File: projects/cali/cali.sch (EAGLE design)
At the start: 25 parts, among them T1 IRLML2502, T2 IRLML2502, T3 2N7002E, T4 IRLML2502

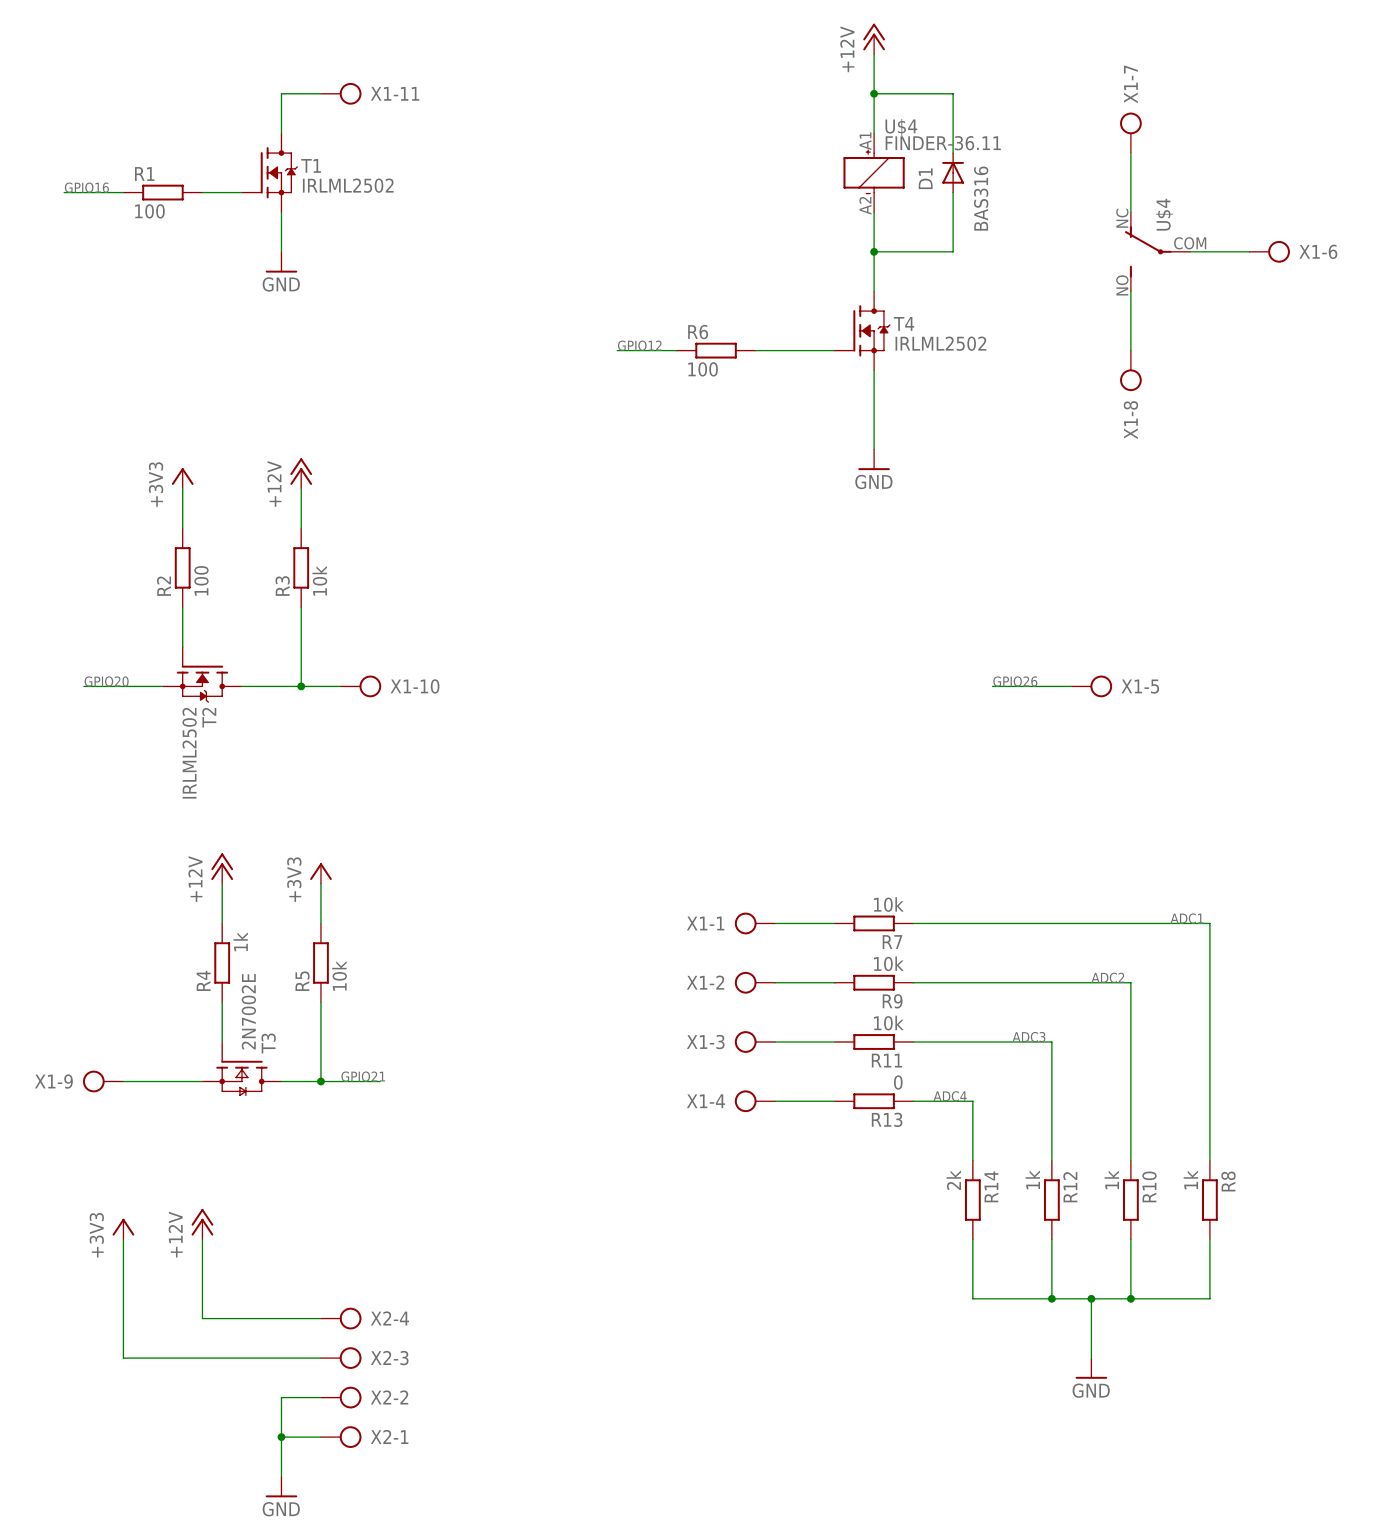
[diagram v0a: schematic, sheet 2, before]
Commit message: Caliboard 1.0 routing done
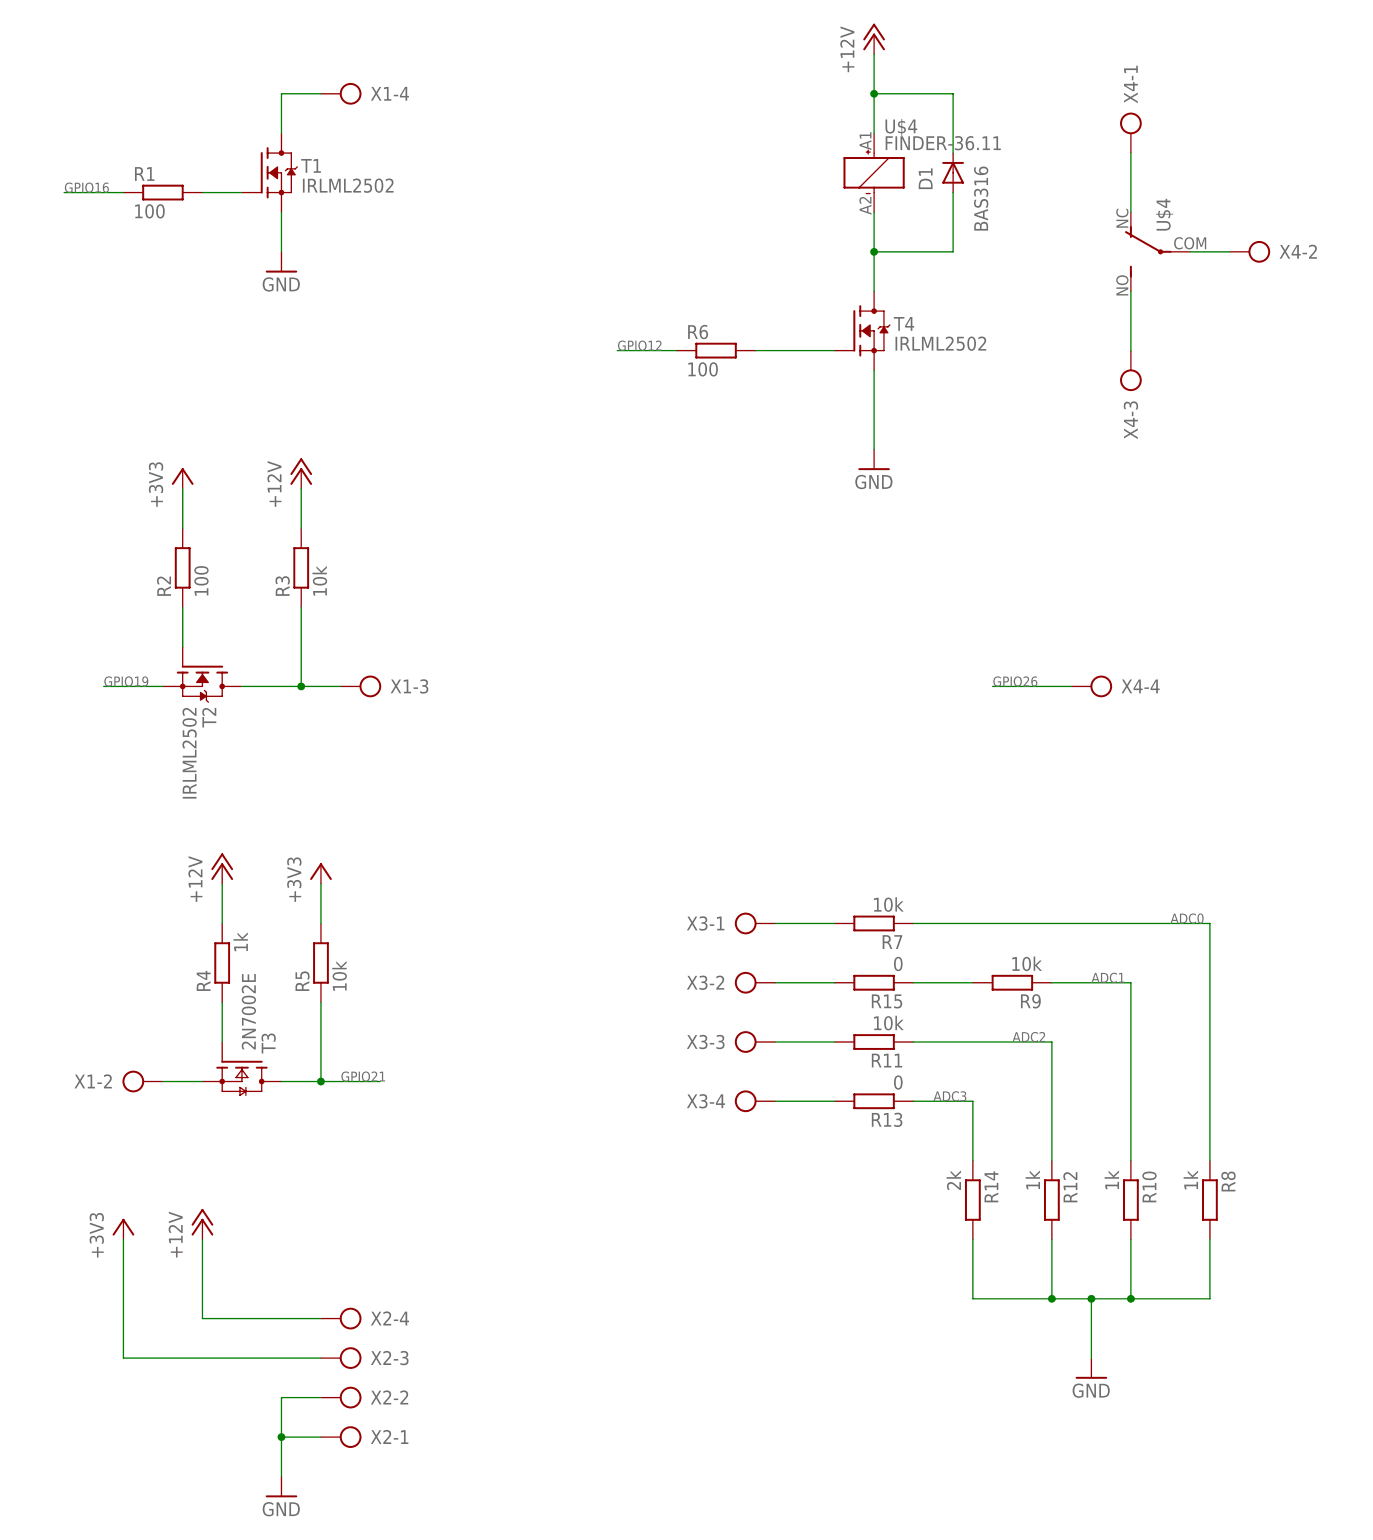
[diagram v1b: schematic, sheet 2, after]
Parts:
- added R15: 0, rcl:R-EU_R1206
- added X3, X4: (no value), con-ptr500:AK500/4
- X1: device con-ptr500:AK500/12 -> con-ptr500:AK500/4
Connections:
- removed net ADC4: R13.1, R14.1
- removed net N$14: R11.2, X1-3.KL
- removed net N$15: R13.2, X1-4.KL
- new net I_SOL: R13.2, X3-4.KL
- new net V_SOL: R7.2, X3-1.KL
- new net V_START: R11.2, X3-3.KL
- net ADC0: now also R7.1, R8.1
- net ADC1: now also R10.1, R9.1; no longer R7.1, R8.1
- net ADC2: now also R11.1, R12.1; no longer R10.1, R9.1
- net ADC3: now also R13.1, R14.1; no longer R11.1, R12.1
- net GPIO19: now also T2.S
- net GPIO20: no longer T2.S
- net GPIO26: now also X4-4.KL; no longer X1-5.KL
- net N$11: now also X1-3.KL; no longer X1-10.KL
- net N$13: now also R15.1, R9.2; no longer T3.S, X1-9.KL
- net N$2: now also X1-4.KL; no longer X1-11.KL
- net N$3: now also X4-3.KL; no longer X1-8.KL
- net N$5: now also X4-2.KL; no longer X1-6.KL
- net N$7: now also X4-1.KL; no longer X1-7.KL
- net N$8: now also T3.S, X1-2.KL; no longer R7.2, X1-1.KL
- net N$9: now also R15.2, X3-2.KL; no longer R9.2, X1-2.KL
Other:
- moved on the sheet: R9, X1-2, X1-3, X1-4
